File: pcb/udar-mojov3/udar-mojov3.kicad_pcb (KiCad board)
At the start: 2 copper layers, 27 parts, among them J1 Conn_02x03_Odd_Even, M1 Motor_Servo_AirTronics, M2 Motor_Servo_AirTronics, Q1 Q_PNP_BCE, Q2 Q_PNP_BCE, Q3 Q_NPN_BCE, SW1 SW_Push, U1 HC-SR04, U2 ZG-Mxx, U3 Mojov3, U4 AP1117-50

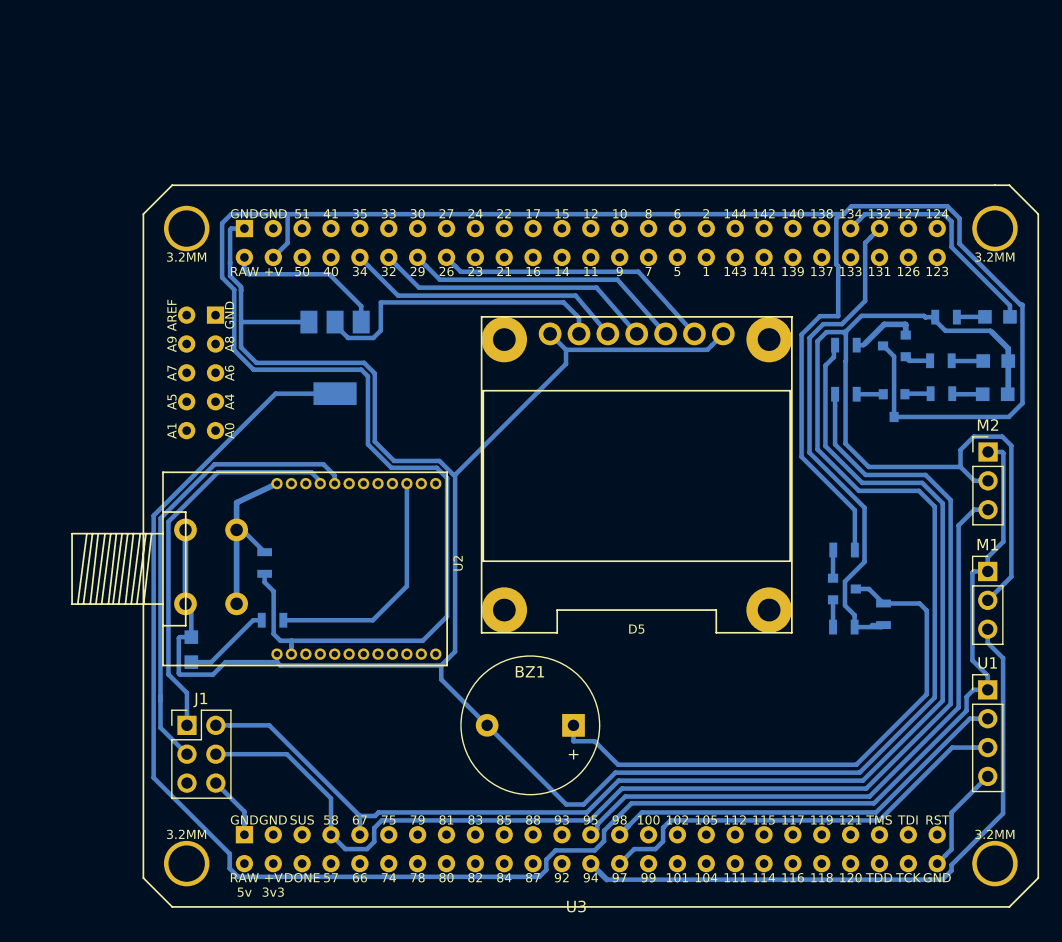
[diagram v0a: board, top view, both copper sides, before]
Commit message: Update;
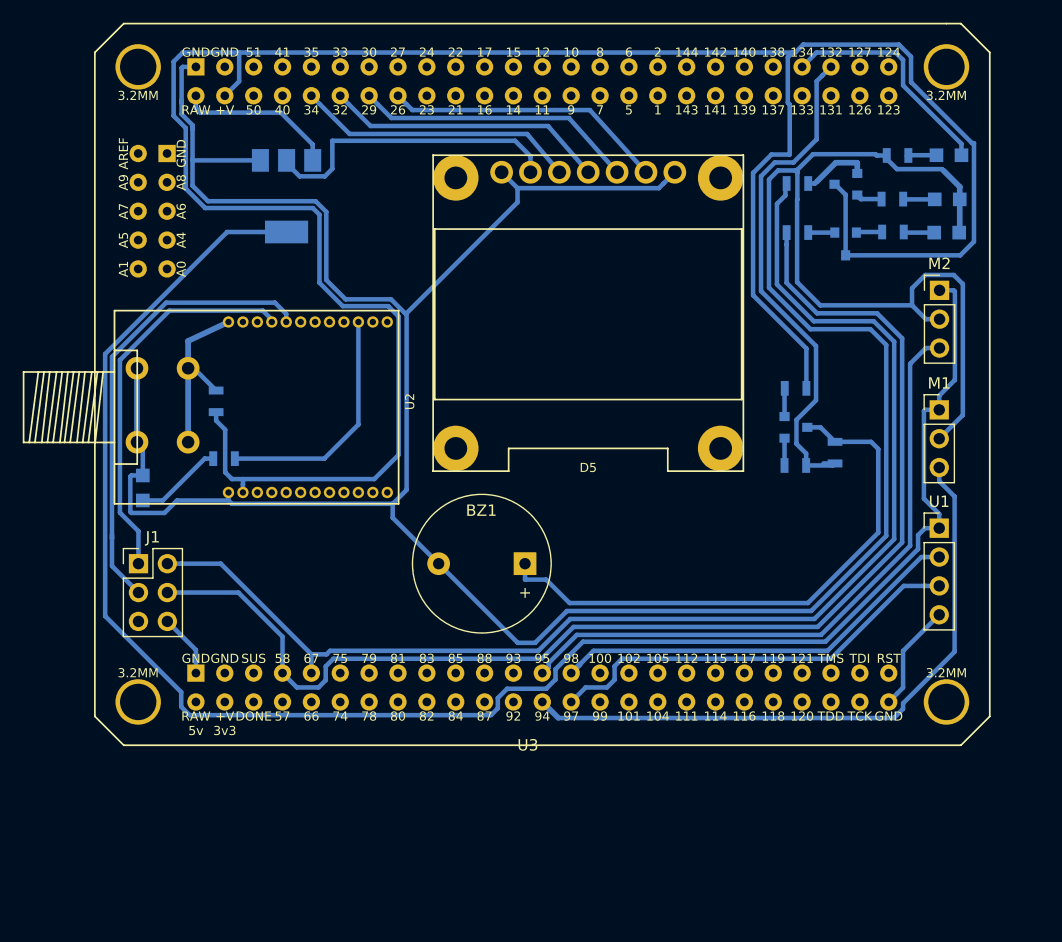
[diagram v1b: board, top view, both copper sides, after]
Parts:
- moved D2 14.9 mm to (181.2, 82.3)
- moved D3 14.9 mm to (181.2, 85.3)
- moved D4 14.9 mm to (181.4, 78.5)
- moved D5 14.9 mm to (149.7, 80.0)
- moved Q1 14.9 mm to (172.3, 81.0)
- moved Q2 14.9 mm to (172.3, 86.3)
- moved Q3 14.9 mm to (167.9, 102.4)
- moved R3 14.9 mm to (168.1, 80.9)
- moved R5 14.9 mm to (168.1, 85.3)
- moved R6 14.9 mm to (176.5, 85.2)
- moved R7 14.9 mm to (167.9, 99.0)
- moved R9 14.9 mm to (171.4, 104.6)
- moved U3 14.9 mm to (144.3, 92.3)
- moved U2 14.9 mm to (119.0, 100.6)
- moved M1 14.9 mm to (180.5, 100.9)
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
